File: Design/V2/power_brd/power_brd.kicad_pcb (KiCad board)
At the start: 4 copper layers, 70 x 75 mm, 54 parts, among them J1 XT60PW-M, J2 Conn_02x03_Odd_Even, J3 Conn_02x04_Odd_Even, J4 Conn_02x04_Odd_Even, U1 TPS5430DDAR, U2 TPS5430DDAR, U3 TPS5430DDAR, U4 TPS5430DDAR, U5 TPS5430DDAR

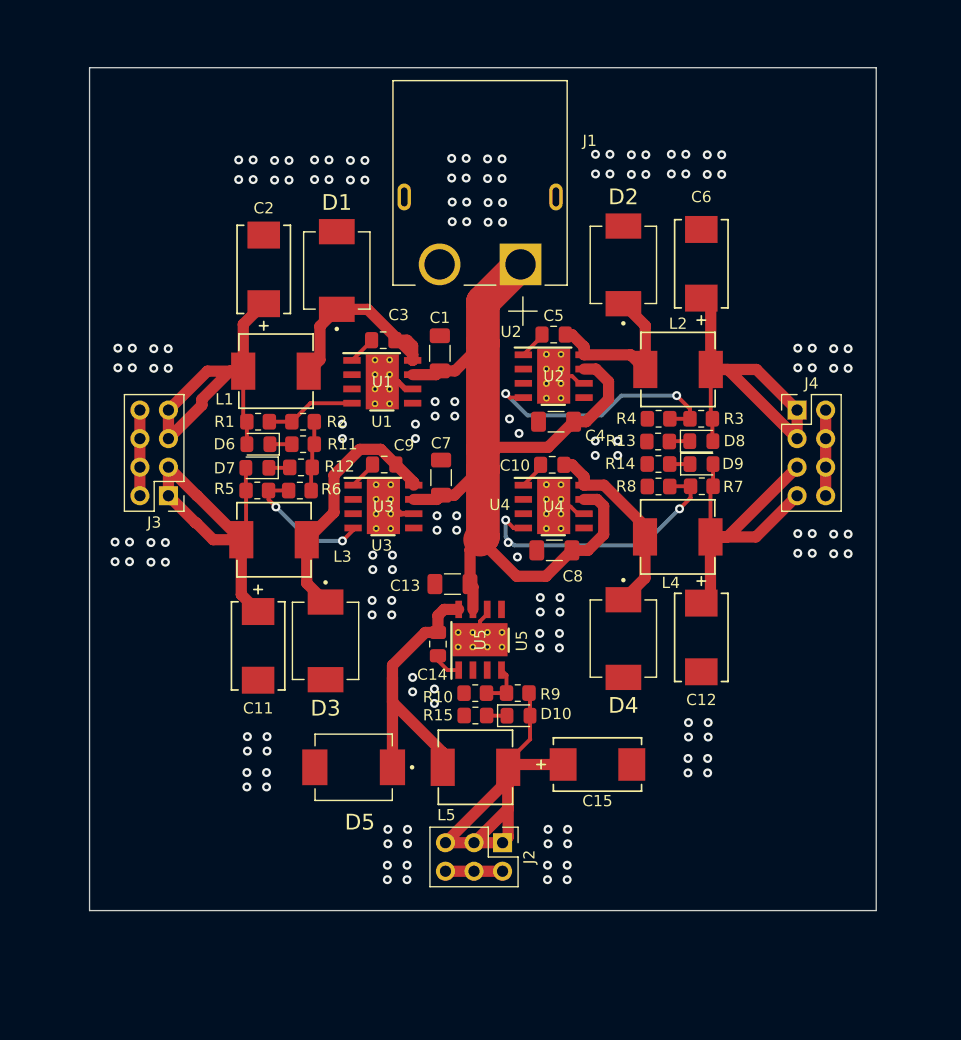
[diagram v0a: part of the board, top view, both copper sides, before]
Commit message: power board
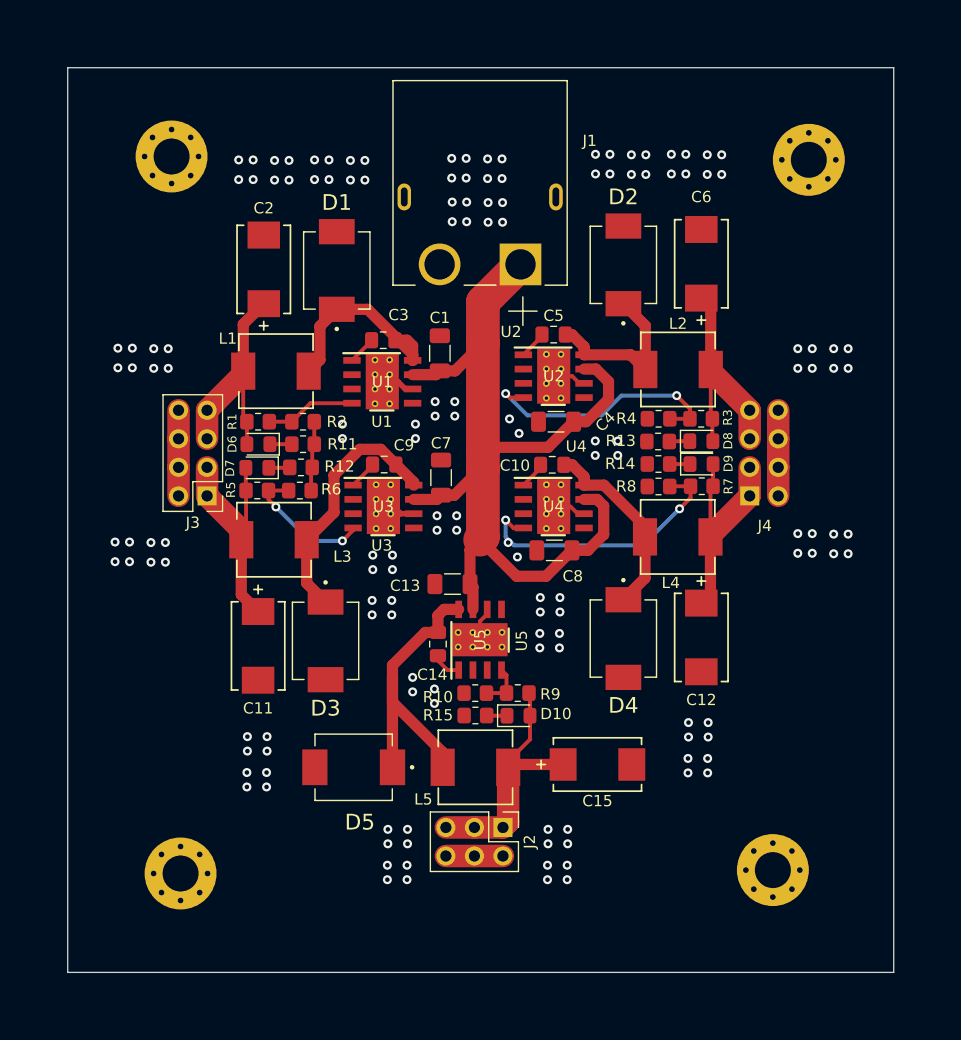
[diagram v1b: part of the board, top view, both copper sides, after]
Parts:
- added H1: MountingHole_Pad, MountingHole:MountingHole_3.2mm_M3_Pad_Via, F.Cu at (90.8, 48.4)
- added H2: MountingHole_Pad, MountingHole:MountingHole_3.2mm_M3_Pad_Via, F.Cu at (91.6, 112.2)
- added H3: MountingHole_Pad, MountingHole:MountingHole_3.2mm_M3_Pad_Via, F.Cu at (144.3, 111.9)
- added H4: MountingHole_Pad, MountingHole:MountingHole_3.2mm_M3_Pad_Via, F.Cu at (147.5, 48.7)
- J4: moved to B.Cu
- moved J4 8.72 mm to (142.2, 78.6)
- moved J3 3.44 mm to (94.0, 78.6)
- moved J2 1.36 mm to (120.3, 108.1)
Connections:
- J4 pad 1: VDD_SERVO_5_6 -> VDD_SERVO_7_8
- J4 pad 3: VDD_SERVO_5_6 -> VDD_SERVO_7_8
- J4 pad 5: VDD_SERVO_7_8 -> VDD_SERVO_5_6
- J4 pad 7: VDD_SERVO_7_8 -> VDD_SERVO_5_6
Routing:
- net VDD_FC: track 41.4 -> 24.2 mm
- net VDD_SERVO_5_6: track 35.1 -> 20.8 mm
- net VDD_SERVO_3_4: track 33.4 -> 21.3 mm
- net VDD_SERVO_7_8: track 32.3 -> 20.4 mm
- net VDD_SERVO_1_2: track 32.3 -> 20.7 mm
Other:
- board size 70 x 75 mm -> 73.5 x 80.5 mm
